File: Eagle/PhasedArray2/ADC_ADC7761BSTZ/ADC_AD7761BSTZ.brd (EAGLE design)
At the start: 65 x 56 mm, 42 parts, among them U1 AD7761BSTZ, Y1 HCM4932768000ABJT

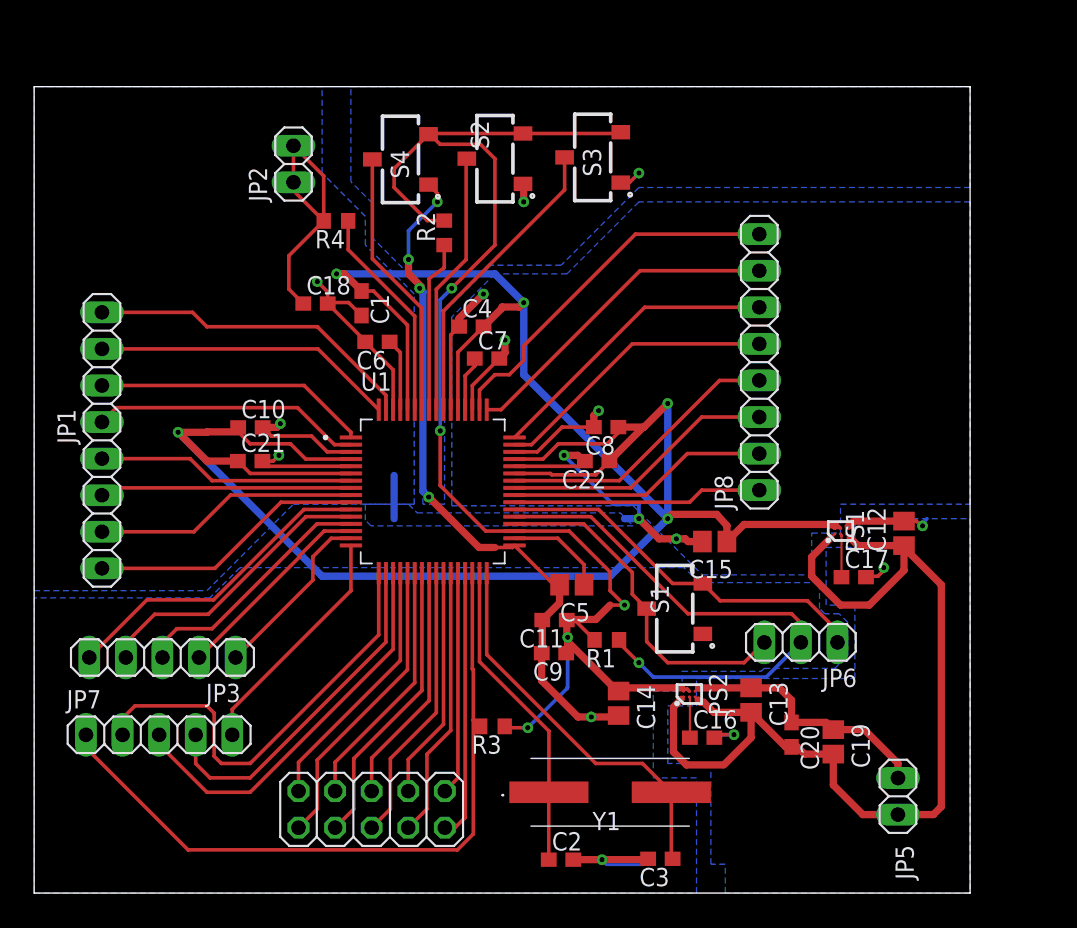
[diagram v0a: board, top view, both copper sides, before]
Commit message: Add files via upload
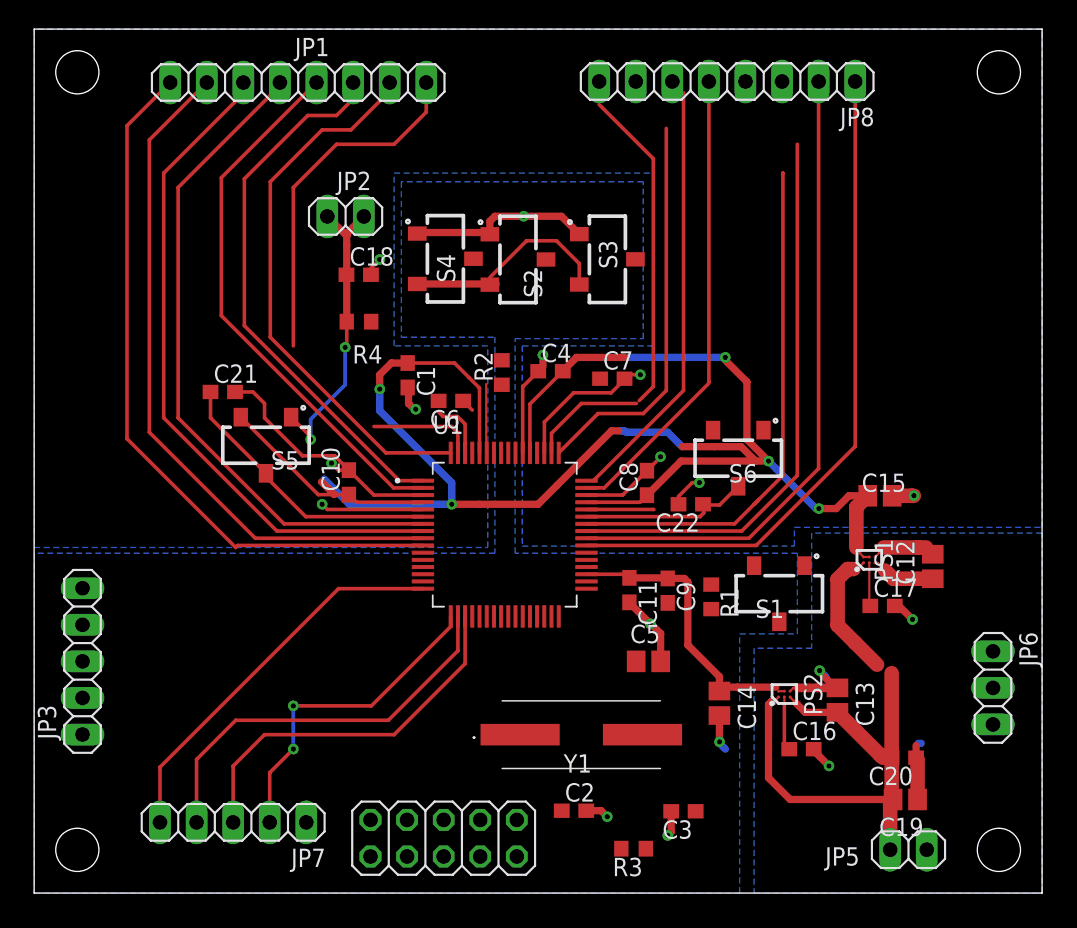
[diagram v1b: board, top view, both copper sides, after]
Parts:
- added S5, S6: CJS-1200TB, CJS-1200TB:B-TYPE
- moved JP1 28.3 mm to (18.3, 56.3), turned to 0 degrees
- moved JP8 19.6 mm to (48.1, 56.4), turned to 180 degrees
- moved JP6 13.7 mm to (66.6, 14.2), turned to 270 degrees
- moved R3 13.0 mm to (41.6, 3.08)
- moved C15 11.9 mm to (58.7, 27.6), turned to 0 degrees
- moved R2 10.5 mm to (32.5, 36.1)
- moved C9 9.01 mm to (44.0, 21.0), turned to 270 degrees
- moved C7 8.81 mm to (40.1, 35.7)
- moved C20 7.96 mm to (60.4, 9.40), turned to 180 degrees
- moved JP7 7.96 mm to (13.8, 4.91), turned to 180 degrees
- moved R1 7.84 mm to (47.0, 20.6), turned to 270 degrees
- moved C10 7.83 mm to (21.9, 28.5), turned to 90 degrees
- moved S4 7.57 mm to (28.6, 44.0), turned to 270 degrees
- moved C5 7.52 mm to (42.7, 16.1), turned to 0 degrees
- moved S1 7.33 mm to (51.8, 20.8), turned to 180 degrees
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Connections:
- new net N$37: C21.1, S5.2, U1.6
- new net VCC/2: C18.1, JP2.1, JP2.2, R4.2, S5.1, S6.1
- net N$36: now also C22.1, S6.2, U1.43; no longer C18.1, JP2.1, JP2.2, R4.2
- net VCC: now also S5.3, S6.3; no longer C21.1, C22.1, U1.43, U1.6
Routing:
- net VDD: track 98.2 -> 34.6 mm, vias 5 -> 0
- net N$35: track 50.0 -> 0.00 mm
- net VCC: track 168.2 -> 126.9 mm
- net N$6: track 39.1 -> 0.00 mm, vias 1 -> 0
- net DGND: track 60.4 -> 23.5 mm, vias 8 -> 5
- net AIN3+: track 19.2 -> 49.7 mm
- net AIN3-: track 18.3 -> 48.0 mm
- net AIN7+: track 17.3 -> 46.8 mm
- net AIN2+: track 17.5 -> 46.8 mm
- net AIN2-: track 17.9 -> 46.3 mm
- net N$7: track 27.1 -> 0.00 mm
- net AIN7-: track 18.2 -> 45.0 mm
- net N$30: track 26.7 -> 0.00 mm
- net N$28: track 24.2 -> 0.00 mm
- net +9V: track 73.1 -> 49.6 mm
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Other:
- board size 65 x 56 mm -> 70 x 60 mm
